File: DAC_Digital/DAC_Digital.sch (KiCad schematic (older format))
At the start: 47 parts, among them J1 +5V_in, J13 Anlg_I2C, J2 DBG_PORT, J3 DSPL_PORT, J4 Out_SPDIF, J5 Conn_02x20_Odd_Even, J6 Conn_01x07, J7 Conn_01x02, J8 Conn_01x02, Q1 2n7002, Q3 FDS4435, Q5 2N7002, Q6 2N7002, U2 PIC18F6722, Y1 10MHz

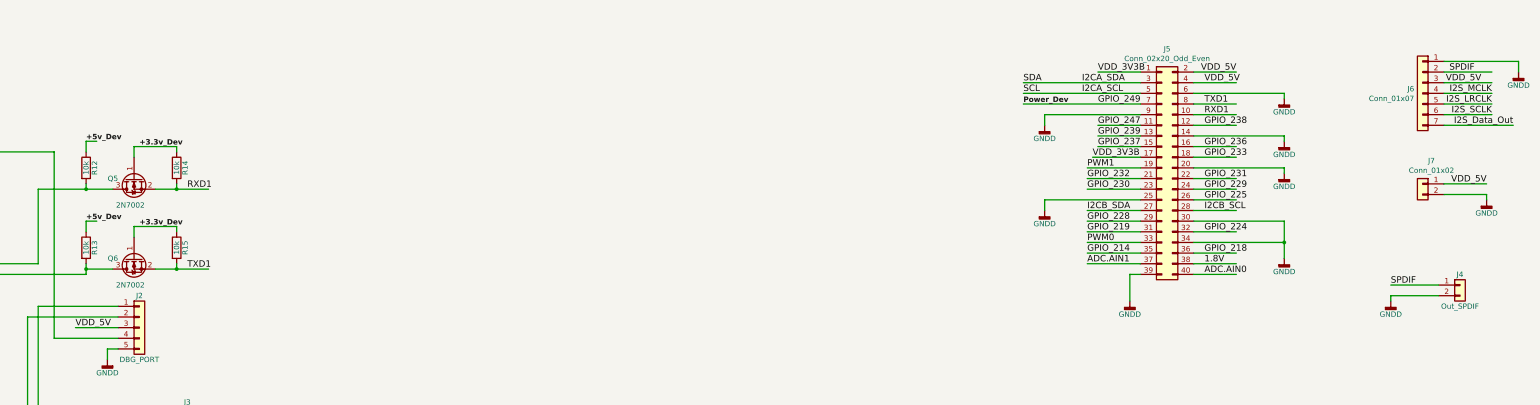
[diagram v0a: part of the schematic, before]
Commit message: Update layout
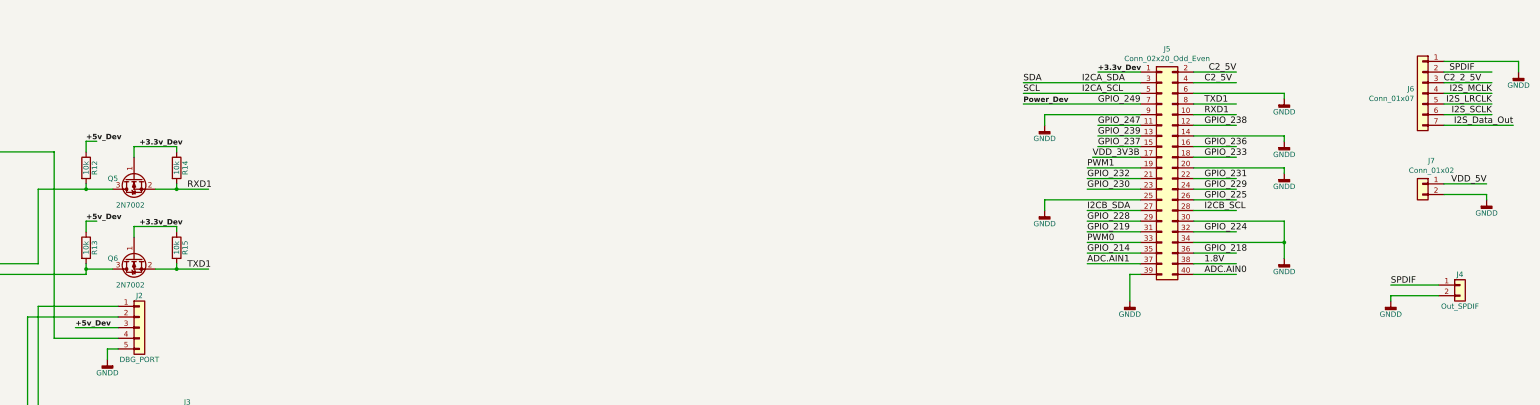
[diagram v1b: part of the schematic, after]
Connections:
- net labels added: C2_2_5V, C2_5V
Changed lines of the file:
@@
 	1    0    0    -1
 $EndComp
-Text Label 17550 1900 0    60   ~ 0
-VDD_3V3B
 Text Label 18850 1900 2    60   ~ 0
-VDD_5V
+C2_5V
 Text Label 18550 2000 0    60   ~ 0
-VDD_5V
+C2_5V
 Text Label 17550 2200 0    60   ~ 0
 GPIO_249
@@
 	1    0    0    -1
 $EndComp
-Text Label 7950 4300 0    60   ~ 0
-VDD_5V
 Connection ~ 4350 2650
 Wire Wire Line
@@
 	20800 2000 21250 2000
 Text Label 21150 2000 2    60   ~ 0
-VDD_5V
+C2_2_5V
 $Comp
 L Connector_Generic:Conn_01x02 J7
@@
 Text Label 8050 3300 0    50   ~ 10
 +5v_Dev
+Text Label 7950 4300 0    50   ~ 10
++5v_Dev
+Text Label 17550 1900 0    50   ~ 10
++3.3v_Dev
 $EndSCHEMATC
